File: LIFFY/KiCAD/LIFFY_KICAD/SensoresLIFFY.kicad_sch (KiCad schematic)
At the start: 26 parts, among them J2 pH, J3 TDS, J4 LDR_CONECTOR, J5 DHT11, J6 LEVEL_SENSOR2, J9 LEVEL_SENSOR1, U1 LM358, U2 LM358, U3 PC817, U5 PC817

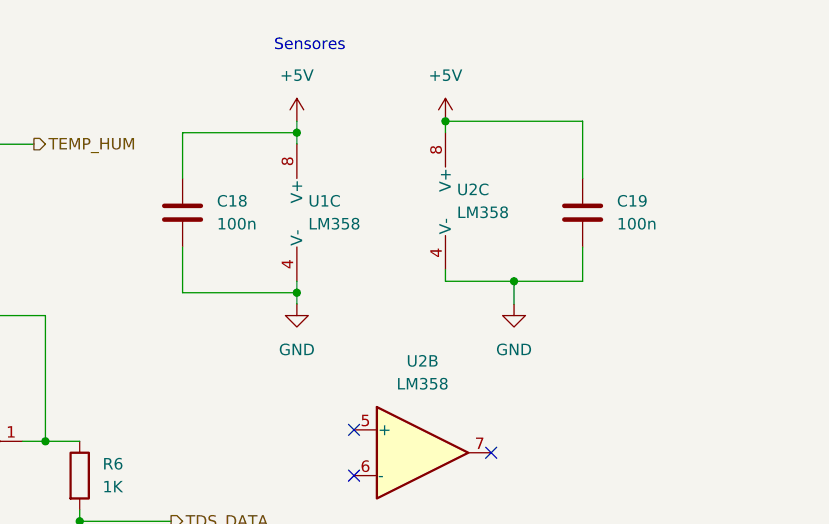
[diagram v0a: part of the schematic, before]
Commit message: V3 Fixed
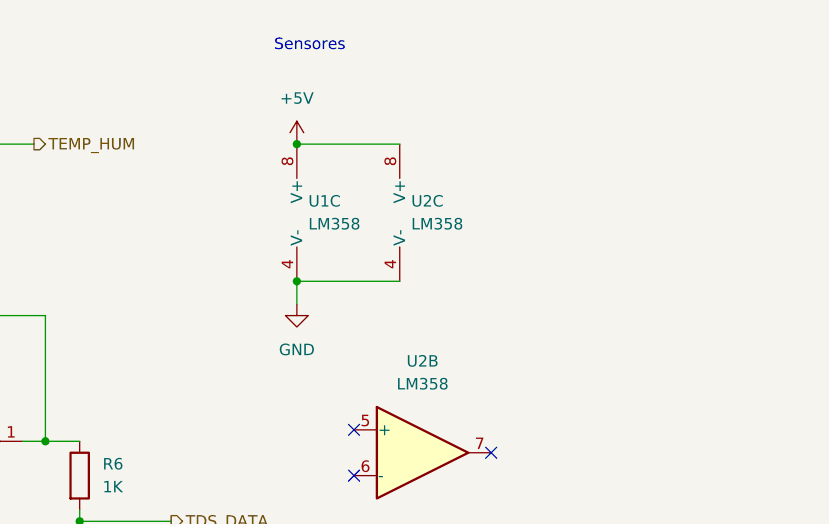
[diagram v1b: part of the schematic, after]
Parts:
- removed C18, C19: 100n, Capacitor_SMD:C_0201_0603Metric, symbol Device:C
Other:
- moved on the sheet: U2C

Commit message: V4.5 Fixed
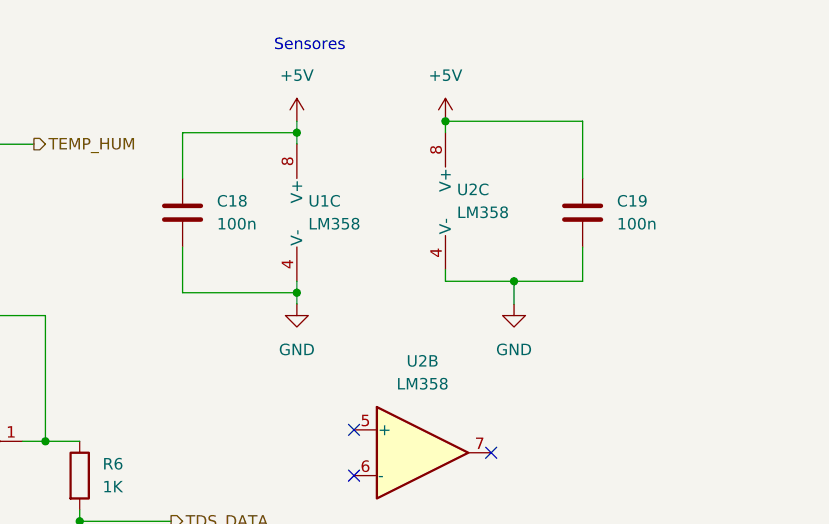
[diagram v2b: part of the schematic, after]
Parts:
- added C18, C19: 100n, Capacitor_SMD:C_0201_0603Metric, symbol Device:C
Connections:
- net +5V: now also C18.1, C19.1
- net GND: now also C18.2, C19.2
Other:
- moved on the sheet: U2C
